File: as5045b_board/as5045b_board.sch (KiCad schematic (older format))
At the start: 21 parts, among them J1 Conn_01x04, J2 Conn_01x04, U1 AS5304, U2 AS5304, U3 LTC3221

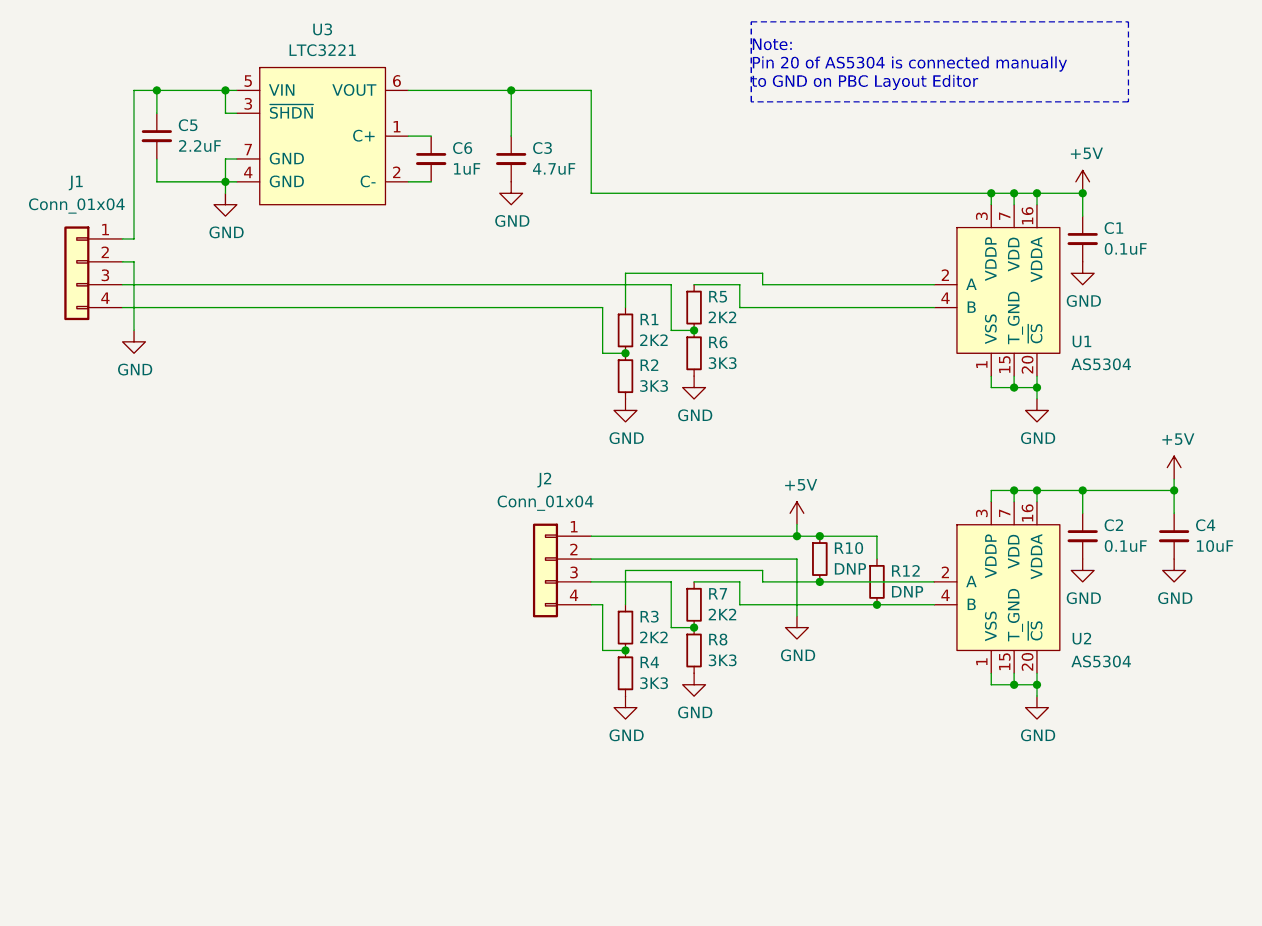
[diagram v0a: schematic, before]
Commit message: Encoders update
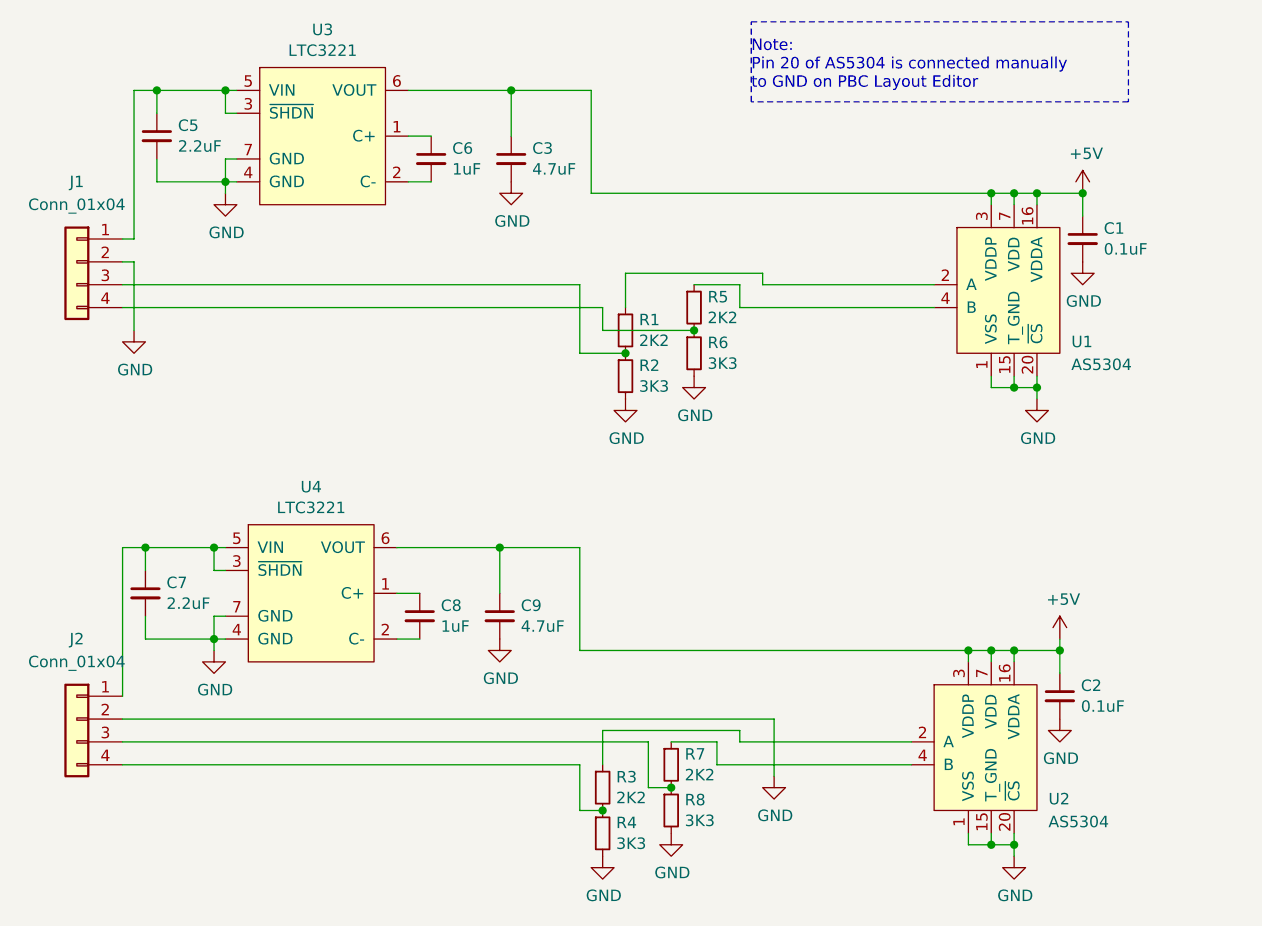
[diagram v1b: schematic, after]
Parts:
- removed C4: 10uF, Capacitor_SMD:C_0603_1608Metric, symbol Device:C_Small
- removed R10, R12: DNP, Resistor_SMD:R_0402_1005Metric, symbol Device:R_Small
- added C7: 2.2uF, Capacitor_SMD:C_0603_1608Metric, symbol Device:C_Small
- added C8: 1uF, Capacitor_SMD:C_0402_1005Metric, symbol Device:C_Small
- added C9: 4.7uF, Capacitor_SMD:C_0603_1608Metric, symbol Device:C_Small
- added U4: LTC3221, Package_DFN_QFN:DFN-6-1EP_2x2mm_P0.5mm_EP0.61x1.42mm, symbol synermycha-electronics:LTC3221
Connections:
- net +5V: now also C9.1, U4.6 (VOUT); no longer J2.1 (Pin_1)
- net GND: now also C7.2, C9.2, U4.4 (GND), U4.7 (GND)
- net at R5.2, R6.1: now also J1.4 (Pin_4); no longer J1.3 (Pin_3)
- net at R1.2, R2.1: now also J1.3 (Pin_3); no longer J1.4 (Pin_4)
- new net: C7.1, J2.1 (Pin_1), U4.3 (~SHDN), U4.5 (VIN)
- new net: C8.1, U4.1 (C+)
- new net: C8.2, U4.2 (C-)
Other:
- moved on the sheet: C2, J2, R3, R4, R7, R8, U2
